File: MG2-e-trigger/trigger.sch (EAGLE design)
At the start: 18 parts, among them IC1 4538D, T1 BC847, T2 BC847

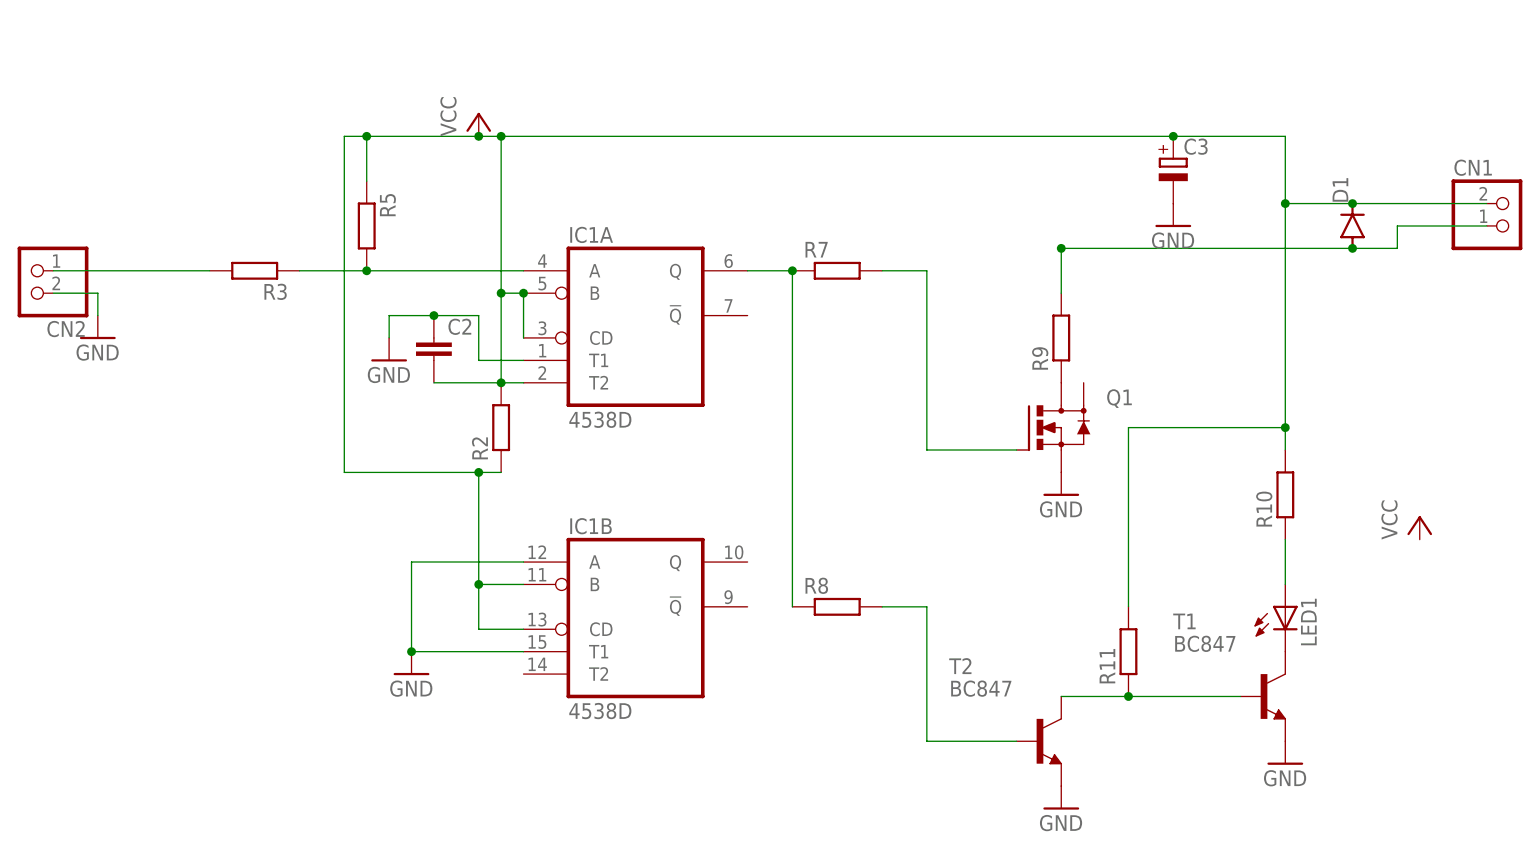
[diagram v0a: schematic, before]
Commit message: trigger change
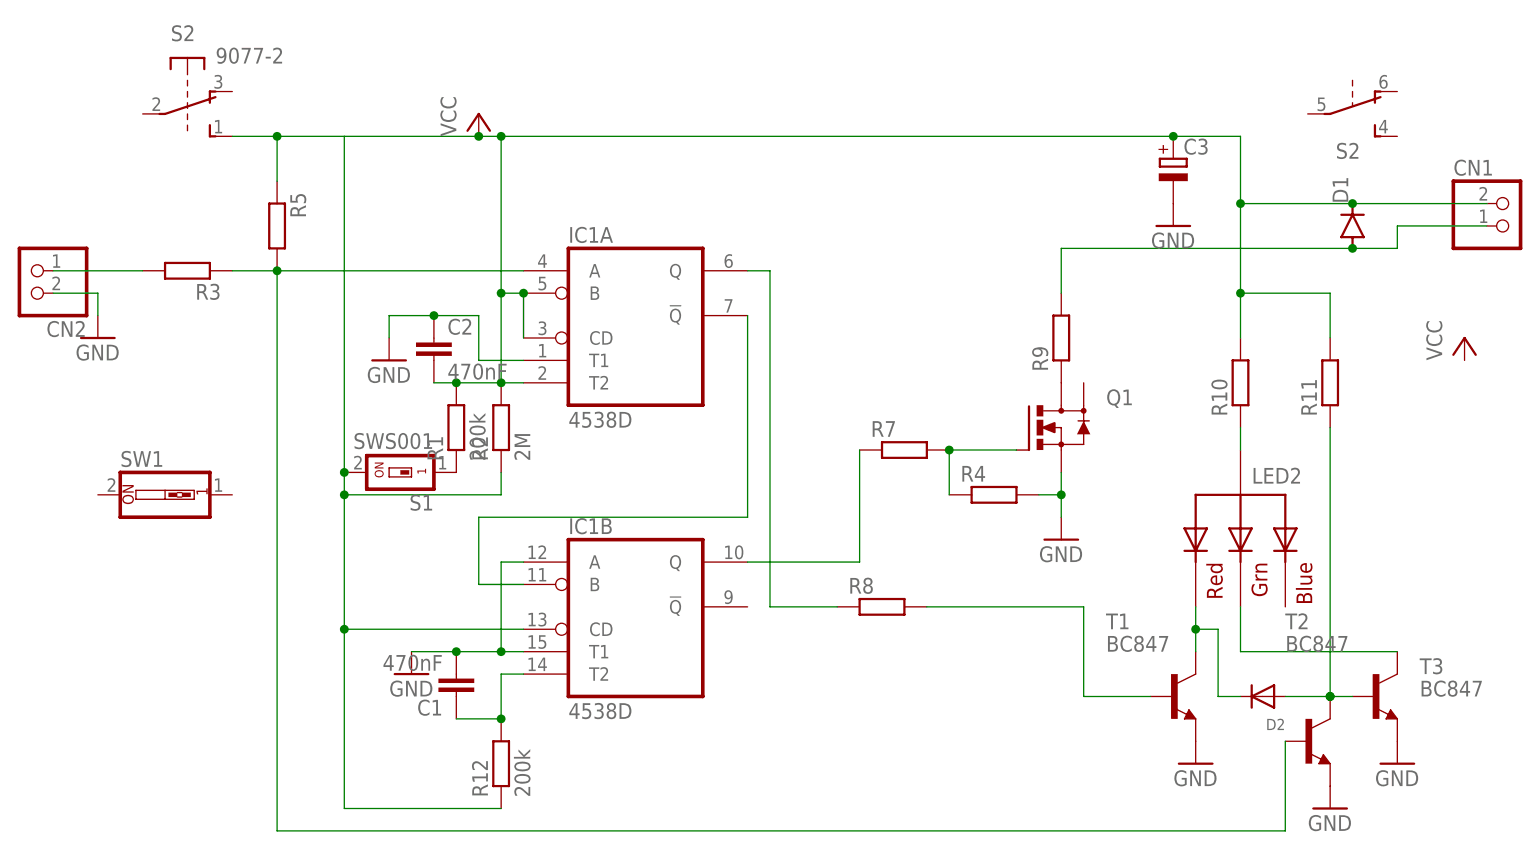
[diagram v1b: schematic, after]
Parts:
- removed LED1: (no value), adafruit:LED3MM
- added C1: 470nF, eagle-ltspice:C
- added D2: (no value), adafruit:DIODESMA
- added LED2: RGBLED_CA-5MM, adafruit:RGBLED_CA-5MM
- added R1, R12: 200k, eagle-ltspice:RR1206
- added R4: (no value), eagle-ltspice:RR1206
- added S1: SWS001, smd-special:SWS001
- added S2: 9077-2, switch-misc:9077-2
- added SW1: (no value), special:SW_DIP-1
- added T3: BC847, transistor:BC847
- C2: value (none) -> 470nF
- R2: value (none) -> 2M
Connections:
- new net N$10: IC1A.Q, R8.1
- new net N$11: LED2.GREEN, T2.C
- new net N$13: IC1A.!Q, IC1B.B
- new net N$14: R1.1, S1.1
- new net N$15: D2.C, LED2.RED, T1.C
- net GND: now also C1.2, R4.2, T3.E
- net N$1: now also C1.1, IC1B.T2, R12.2; no longer LED1.C, T1.C
- net N$12: now also R4.1
- net N$3: now also T3.B
- net N$4: now also IC1B.Q; no longer IC1A.Q, R8.1
- net N$6: now also D2.A, R11.1, T3.C; no longer R8.2
- net N$8: now also R8.2; no longer R11.1, T2.C
- net N$9: now also LED2.VCC; no longer LED1.A
- net VCC: now also R1.2, R12.1, S1.2, S21.S; no longer IC1B.B
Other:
- moved on the sheet: R10, R11, R3, R5, R7, R8, T1, T2
